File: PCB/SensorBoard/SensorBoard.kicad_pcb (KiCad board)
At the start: 2 copper layers, 99.1 x 30.5 mm, 16 parts, among them J1 Conn_02x04_Odd_Even, U1 TCRT5000, U2 TCRT5000, U3 TCRT5000, U4 TCRT5000, U5 TCRT5000

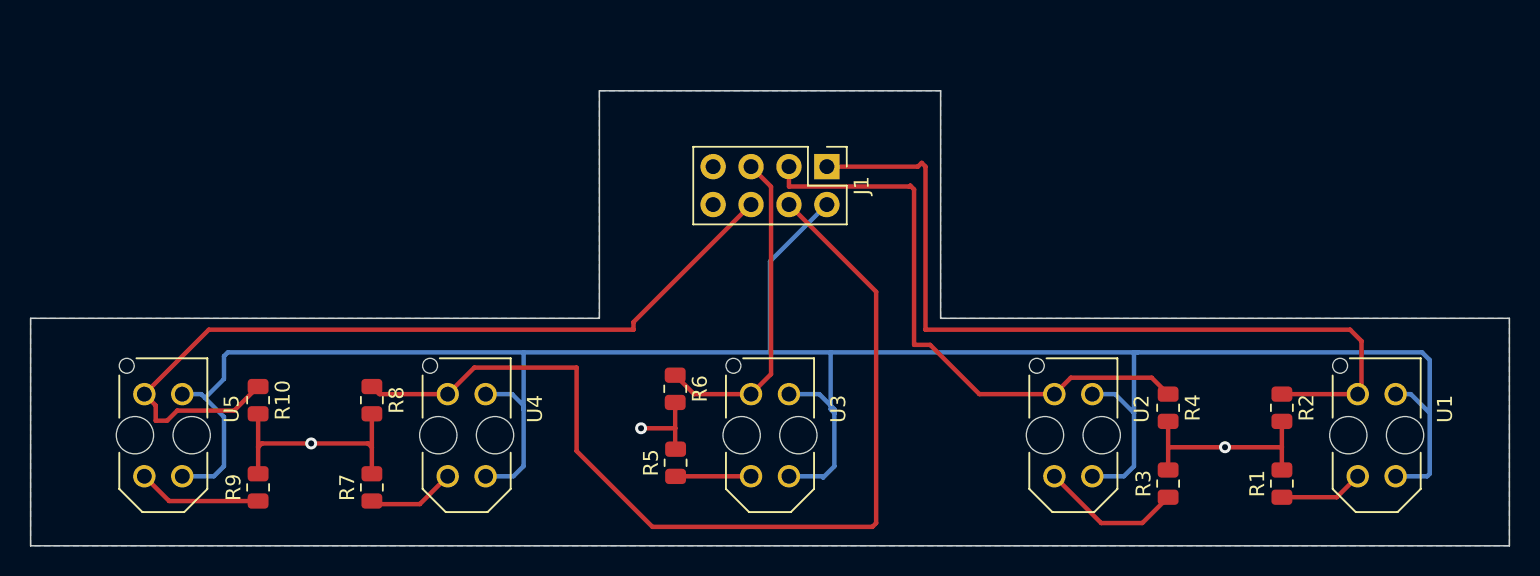
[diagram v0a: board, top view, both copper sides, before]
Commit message: Cleaned up repo
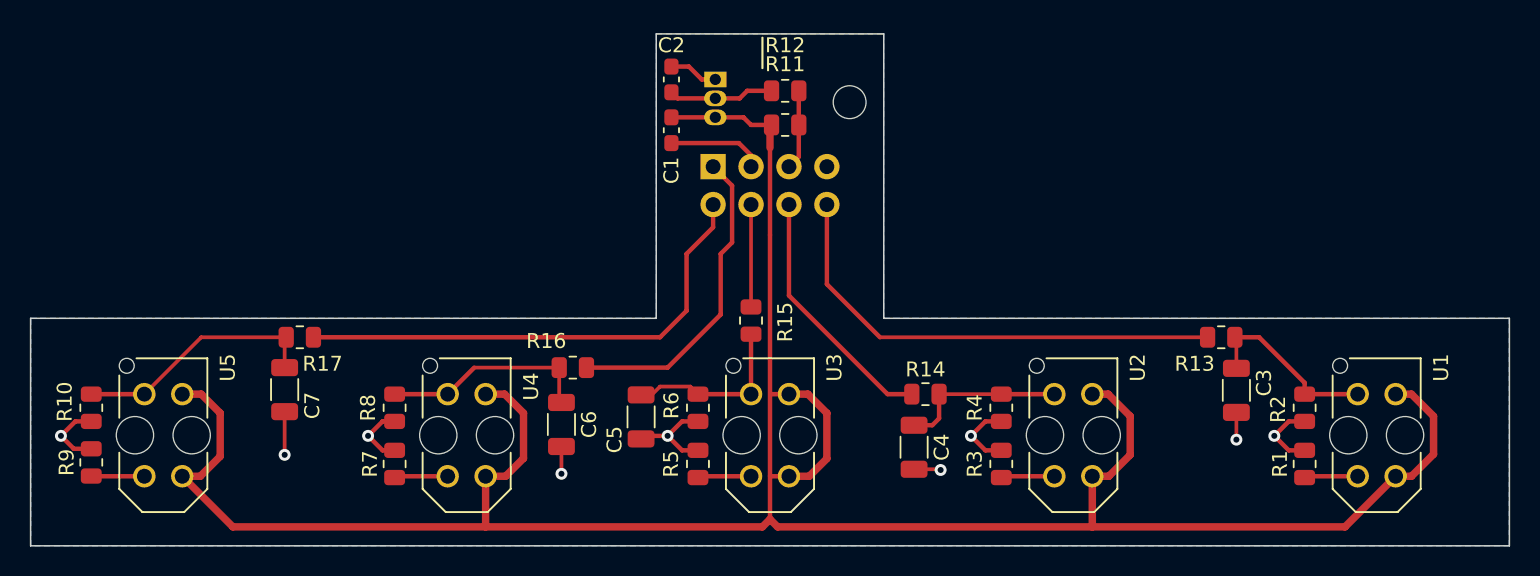
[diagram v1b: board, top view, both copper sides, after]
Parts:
- added C1: 1u, Capacitor_SMD:C_0603_1608Metric_Pad1.08x0.95mm_HandSolder, F.Cu at (144.5, 48.4)
- added C2: 1u, Capacitor_SMD:C_0603_1608Metric_Pad1.08x0.95mm_HandSolder, F.Cu at (144.5, 45.0)
- added C3: C, Capacitor_SMD:C_1206_3216Metric, F.Cu at (182.4, 65.8)
- added C4: C, Capacitor_SMD:C_1206_3216Metric, F.Cu at (160.8, 69.6)
- added C5: C, Capacitor_SMD:C_1206_3216Metric, F.Cu at (142.5, 67.6)
- added C6: C, Capacitor_SMD:C_1206_3216Metric, F.Cu at (137.2, 68.1)
- added C7: C, Capacitor_SMD:C_1206_3216Metric, F.Cu at (118.6, 65.7)
- added H1: MountingHole, MountingHole:MountingHole_2.2mm_M2, F.Cu at (156.5, 46.5)
- added R11: 0R, Resistor_SMD:R_0805_2012Metric, F.Cu at (152.1, 48.0)
- added R12: 0R, Resistor_SMD:R_0805_2012Metric, F.Cu at (152.1, 45.7)
- added R13: R, Resistor_SMD:R_0805_2012Metric, F.Cu at (181.4, 62.2)
- added R14: R, Resistor_SMD:R_0805_2012Metric, F.Cu at (161.5, 66.0)
- added R15: R, Resistor_SMD:R_0805_2012Metric, F.Cu at (149.9, 61.1)
- added R16: R, Resistor_SMD:R_0805_2012Metric, F.Cu at (137.9, 64.3)
- added R17: R, Resistor_SMD:R_0805_2012Metric, F.Cu at (119.6, 62.2)
- added U6: MCP1700x-330xxTO, Package_TO_SOT_THT:TO-92_Inline, B.Cu at (147.5, 45.0)
- J1: value Conn_02x04_Odd_Even -> IR Bridge Connector; moved to B.Cu
- U1, U2, U3, U4, U5: footprint kicad_mod:OPTO_TCRT5000 -> OptoDevice:OPTO_TCRT5000
- moved R9 11.3 mm to (105.7, 70.6)
- moved R3 11.3 mm to (166.6, 70.7)
- moved R10 11.2 mm to (105.7, 67.0)
- moved R4 11.2 mm to (166.6, 67.0)
- moved J1 7.62 mm to (147.3, 50.8)
- moved R7 2.19 mm to (126.0, 70.7)
- moved R1 2.01 mm to (186.9, 70.7)
- moved R6 1.98 mm to (146.3, 67.0)
- moved R8 1.61 mm to (126.0, 67.0)
- moved R2 1.52 mm to (186.9, 67.0)
- moved R5 1.50 mm to (146.3, 70.7)
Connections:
- J1 pad 1: Analog Pin1 -> /Sense_4
- J1 pad 2: +3.3V -> /Sense_5
- J1 pad 3: Analog Pin2 -> GND
- J1 pad 4: Analog Pin4 -> /Sense_3
- J1 pad 5: Analog Pin3 -> Net-(J1-Pin_5)
- J1 pad 6: Analog Pin5 -> /Sense_2
- J1 pad 8: unconnected-(J1-Pin_8-Pad8) -> /Sense_1
- R10 pad 1: Analog Pin5 -> /Sense_5_R
- R2 pad 1: Analog Pin1 -> /Sense_1_R
- R4 pad 1: Analog Pin2 -> /Sense_2_R
- R6 pad 1: Analog Pin3 -> /Sense_3_R
- R8 pad 1: Analog Pin4 -> /Sense_4_R
- U1 pad E: Analog Pin1 -> /Sense_1_R
- U2 pad E: Analog Pin2 -> /Sense_2_R
- U3 pad E: Analog Pin3 -> /Sense_3_R
- U4 pad E: Analog Pin4 -> /Sense_4_R
- U5 pad E: Analog Pin5 -> /Sense_5_R
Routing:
- net Analog Pin4: track 67.0 -> 0.00 mm
- net Analog Pin5: track 56.1 -> 0.00 mm
- net Analog Pin1: track 56.0 -> 0.00 mm
- net Analog Pin2: track 39.6 -> 0.00 mm
- net /Sense_5: track 0.00 -> 33.6 mm
- net /Sense_1: track 0.00 -> 32.3 mm
- net Analog Pin3: track 22.0 -> 0.00 mm
- net /Sense_4: track 0.00 -> 21.2 mm
- net /Sense_2: track 0.00 -> 17.1 mm
- net /Sense_5_R: track 0.00 -> 16.7 mm
- net /Sense_4_R: track 0.00 -> 14.2 mm
- net /Sense_1_R: track 0.00 -> 12.4 mm
- net /Sense_3_R: track 0.00 -> 11.8 mm
- net +3.3V: track 160.9 -> 172.2 mm
- net /Sense_2_R: track 0.00 -> 11.2 mm
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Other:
- board size 99.1 x 30.5 mm -> 99.1 x 34.3 mm
